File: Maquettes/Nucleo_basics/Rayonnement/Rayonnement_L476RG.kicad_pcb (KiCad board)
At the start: 2 copper layers, 120 x 110 mm, 48 parts, among them CON1 MikroE-Accelero, CON2 MikroE-nRF-S-module, J1 Speed_R, J10 Morpho_Gauche, J11 Morpho_Droite, J12 LED_1, J13 LED_2, J14 LED_3, J15 LED_4, J17 I2C_Visu, J18 I2C_EXT, J19 GND_reg, J2 Speed_L, J20 3.3V_reg, J21 MOT_R, J22 MOT_L, J23 D_IN_OUT, J3 Line_R, J4 Line_C, J5 Line_L, J6 US_Sensor, J7 Servo, J8 BAT_IN, J9 TC74A2-TempI2C, SW1 SW_1, SW2 SW_2, U1 MCP9700-Temp, U2 LM7805_TO220, U3 SN754410NE

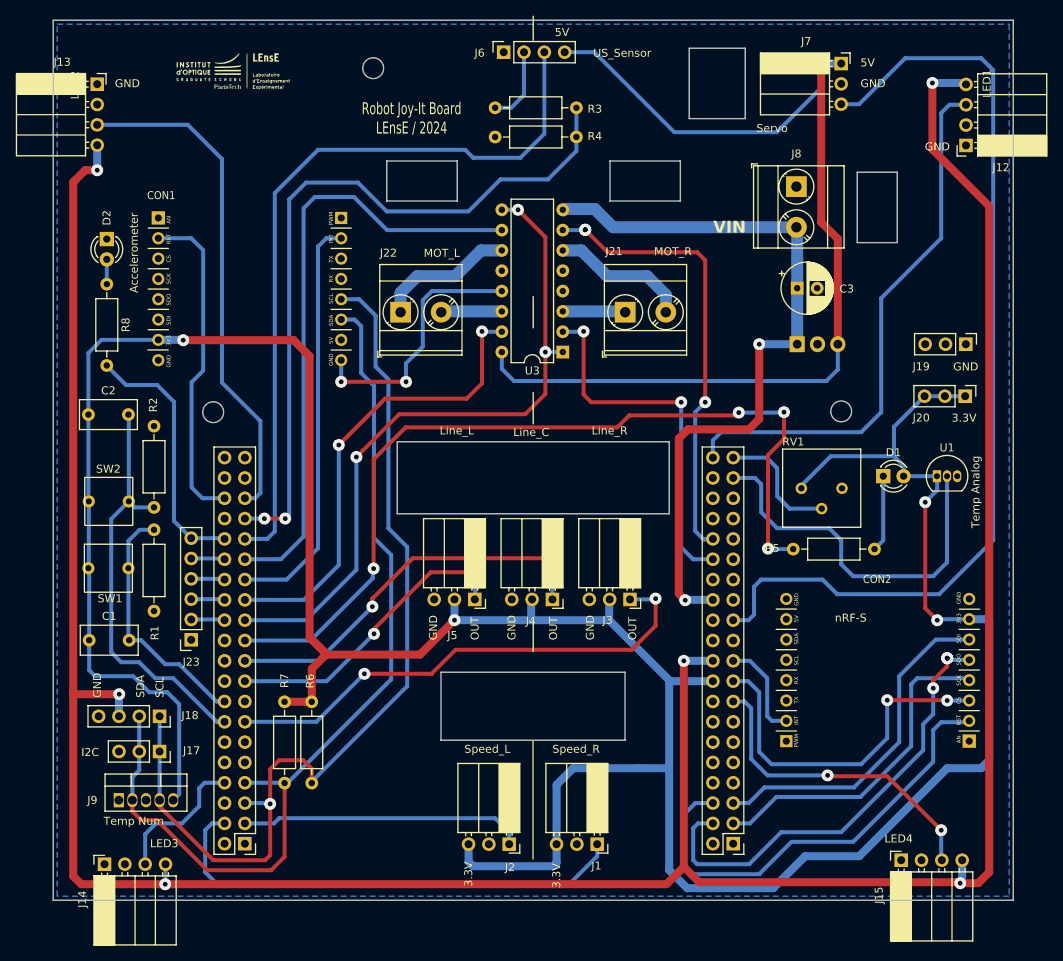
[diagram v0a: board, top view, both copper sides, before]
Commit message: Update Rayonnement
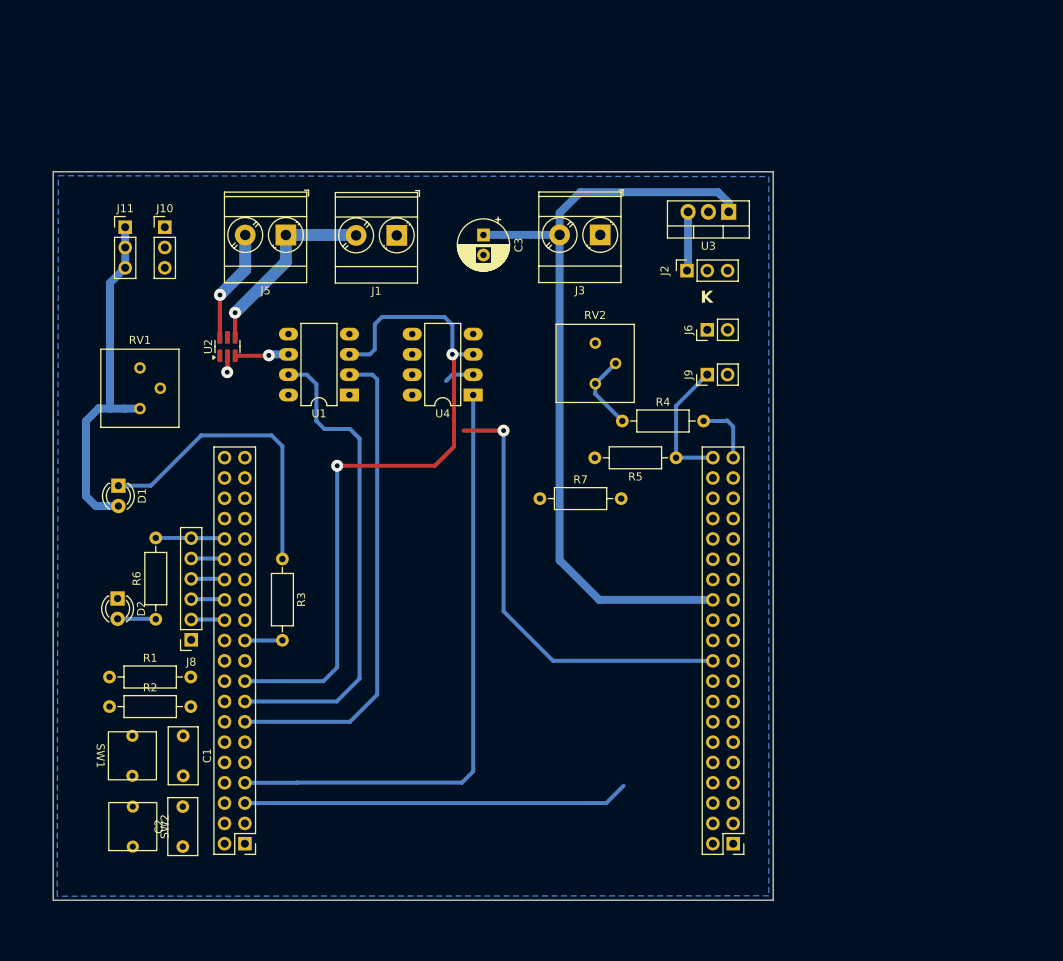
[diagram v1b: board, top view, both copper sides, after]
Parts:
- removed ? (x2): , 
- removed CON1: MikroE-Accelero, mikroE:MIKROBUS_MODULE_CONN
- removed CON2: MikroE-nRF-S-module, mikroE:MIKROBUS_MODULE_CONN
- removed G***: LOGO, LEnsE:Logo_Small
- removed J12: LED_1, Connector_PinSocket_2.54mm:PinSocket_1x04_P2.54mm_Horizontal
- removed J13: LED_2, Connector_PinSocket_2.54mm:PinSocket_1x04_P2.54mm_Horizontal
- removed J14: LED_3, Connector_PinSocket_2.54mm:PinSocket_1x04_P2.54mm_Horizontal
- removed J15: LED_4, Connector_PinSocket_2.54mm:PinSocket_1x04_P2.54mm_Horizontal
- removed J17: I2C_Visu, Connector_PinSocket_2.54mm:PinSocket_1x03_P2.54mm_Vertical
- removed J18: I2C_EXT, Connector_PinSocket_2.54mm:PinSocket_1x04_P2.54mm_Vertical
- removed J19: GND_reg, Connector_PinHeader_2.54mm:PinHeader_1x03_P2.54mm_Vertical
- removed J20: 3.3V_reg, Connector_PinHeader_2.54mm:PinHeader_1x03_P2.54mm_Vertical
- removed J21: MOT_R, TerminalBlock_Phoenix:TerminalBlock_Phoenix_MKDS-3-2-5.08_1x02_P5.08mm_Horizontal
- removed J22: MOT_L, TerminalBlock_Phoenix:TerminalBlock_Phoenix_MKDS-3-2-5.08_1x02_P5.08mm_Horizontal
- removed the J4 at (185.9, 112.9)
- removed the J7 at (222.0, 45.9)
- removed the J8 at (216.4, 61.3)
- removed R8: 100, Resistor_THT:R_Axial_DIN0207_L6.3mm_D2.5mm_P10.16mm_Horizontal
- removed REF** (x2): MountingHole_2.2mm_M2, MountingHole:MountingHole_2.2mm_M2
- added J10: GND_reg, Connector_PinHeader_2.54mm:PinHeader_1x03_P2.54mm_Vertical, F.Cu at (137.4, 66.4)
- added J11: 3.3V_reg, Connector_PinHeader_2.54mm:PinHeader_1x03_P2.54mm_Vertical, F.Cu at (132.5, 66.4)
- added RV2: 100k, Potentiometer_THT:Potentiometer_Bourns_3386P_Vertical, F.Cu at (191.3, 85.9)
- added U4: ~, Package_DIP:DIP-8_W7.62mm_LongPads, F.Cu at (176.0, 87.3)
- J1: value Speed_R -> LED_IN; footprint Connector_PinSocket_2.54mm:PinSocket_1x03_P2.54mm_Horizontal -> TerminalBlock_Phoenix:TerminalBlock_Phoenix_MKDS-3-2-5.08_1x02_P5.08mm_Horizontal
- J2: value Speed_L -> Servo; footprint Connector_PinSocket_2.54mm:PinSocket_1x03_P2.54mm_Horizontal -> Connector_PinSocket_2.54mm:PinSocket_1x03_P2.54mm_Vertical
- J3: value Line_R -> POWER_IN; footprint Connector_PinSocket_2.54mm:PinSocket_1x03_P2.54mm_Horizontal -> TerminalBlock_Phoenix:TerminalBlock_Phoenix_MKDS-3-2-5.08_1x02_P5.08mm_Horizontal
- J5: value Line_L -> LED_OUT; footprint Connector_PinSocket_2.54mm:PinSocket_1x03_P2.54mm_Horizontal -> TerminalBlock_Phoenix:TerminalBlock_Phoenix_MKDS-3-2-5.08_1x02_P5.08mm_Horizontal
- J6: value US_Sensor -> PhotoDiode; footprint Connector_PinSocket_2.54mm:PinSocket_1x04_P2.54mm_Vertical -> Connector_PinHeader_2.54mm:PinHeader_1x02_P2.54mm_Vertical
- J9: value TC74A2-TempI2C -> Thermistance; footprint Package_TO_SOT_THT:TO-220-5_Vertical -> Connector_PinHeader_2.54mm:PinHeader_1x02_P2.54mm_Vertical
- R3: value 2.2k -> 100
- R4: value 3.3k -> 100k
- R5: value 100 -> 10k
- R6: value 680 -> 100
- R7: value 680 -> 1k
- U1: value MCP9700-Temp -> ~; footprint Package_TO_SOT_THT:TO-92_Inline -> Package_DIP:DIP-8_W7.62mm_LongPads
- U2: value LM7805_TO220 -> BCR430UW6; footprint Package_TO_SOT_THT:TO-220-3_Vertical -> Package_TO_SOT_SMD:SC-74-6_1.55x2.9mm_P0.95mm; moved to F.Cu
- U3: value SN754410NE -> LM7805_TO220; footprint Package_DIP:DIP-16_W7.62mm -> Package_TO_SOT_THT:TO-220-3_Vertical
- moved D1 95.6 mm to (131.7, 98.7), turned to -90 degrees
- moved J9 90.8 mm to (205.3, 84.8), turned to 90 degrees
- moved RV1 83.3 mm to (134.3, 89.0), turned to 0 degrees
- moved J1 80.1 mm to (166.4, 67.4), turned to 180 degrees
- moved J2 75.1 mm to (202.7, 71.8), turned to 90 degrees
- moved U1 74.1 mm to (160.5, 87.3), turned to 180 degrees
- moved U2 71.2 mm to (145.3, 81.3), turned to 90 degrees
- moved R3 67.3 mm to (152.2, 107.8), turned to -90 degrees
- moved C2 55.3 mm to (139.7, 143.8), turned to 90 degrees
- moved J5 51.3 mm to (152.6, 67.3), turned to 180 degrees
- moved J3 45.7 mm to (191.9, 67.3), turned to 180 degrees
- moved D2 45.0 mm to (131.6, 112.8)
- moved J6 43.0 mm to (205.3, 79.2)
- moved R7 40.8 mm to (184.3, 100.3), turned to 0 degrees
- moved C3 39.8 mm to (177.3, 67.3), turned to -90 degrees
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- renumbered J10 to J4, J11 to J7, J23 to J8
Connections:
- J1 pad 1: Speed_R -> GND
- J1 pad 2: GND -> LED_POW_IN
- J2 pad 1: Speed_L -> 5V
- J2 pad 3: 3.3V_NUC -> Servo
- J3 pad 1: Line_R -> GND
- J3 pad 2: 3.3V_NUC -> VIN
- J4 pad 15: Din_4 -> unconnected-(J4-Pin_15-Pad15)
- J4 pad 17: nRF_CS -> unconnected-(J4-Pin_17-Pad17)
- J4 pad 19: nRF_INT -> unconnected-(J4-Pin_19-Pad19)
- J4 pad 23: Servo -> unconnected-(J4-Pin_23-Pad23)
- J4 pad 3: SCK -> unconnected-(J4-Pin_3-Pad3)
- J4 pad 30: MOT_R_1 -> POT_OUT
- J4 pad 32: MOT_R_2 -> unconnected-(J4-Pin_32-Pad32)
- J4 pad 34: ADC_OUT -> unconnected-(J4-Pin_34-Pad34)
- J4 pad 36: unconnected-(J10-Pin_36-Pad36) -> POT_NUM_OUT
- J4 pad 37: TEMP_OUT -> unconnected-(J4-Pin_37-Pad37)
- J4 pad 39: POT_OUT -> PHD_OUT
- J4 pad 4: MISO -> unconnected-(J4-Pin_4-Pad4)
- J4 pad 40: Din_1 -> RT_OUT
- J4 pad 5: MOSI -> unconnected-(J4-Pin_5-Pad5)
- J4 pad 6: nRF_CE -> unconnected-(J4-Pin_6-Pad6)
- J5 pad 1: Line_L -> LED_POW_IN
- J5 pad 2: 3.3V_NUC -> Net-(J5-Pin_2)
- J6 pad 1: GND -> 3.3V_NUC
- J6 pad 2: US_echo -> PHD_OUT
- J7 pad 13: Line_R -> SCK
- J7 pad 14: SW2_OUT -> unconnected-(J7-Pin_14-Pad14)
- J7 pad 15: unconnected-(J11-Pin_15-Pad15) -> MISO
- J7 pad 16: SW1_OUT -> unconnected-(J7-Pin_16-Pad16)
- J7 pad 17: Line_L -> MOSI
- J7 pad 19: Line_C -> unconnected-(J7-Pin_19-Pad19)
- J7 pad 23: MOT_EN -> unconnected-(J7-Pin_23-Pad23)
- J7 pad 25: MOT_L_2 -> unconnected-(J7-Pin_25-Pad25)
- J7 pad 27: Accel_INT -> unconnected-(J7-Pin_27-Pad27)
- J7 pad 29: MOT_L_1 -> unconnected-(J7-Pin_29-Pad29)
- J7 pad 3: Speed_L -> unconnected-(J7-Pin_3-Pad3)
- J7 pad 31: US_trig -> CS_1
- J7 pad 33: US_echo_in -> unconnected-(J7-Pin_33-Pad33)
- J7 pad 35: Din_2 -> unconnected-(J7-Pin_35-Pad35)
- J7 pad 36: Accel_RESET -> unconnected-(J7-Pin_36-Pad36)
- J7 pad 4: Speed_R -> SW2_OUT
- J7 pad 5: SCL -> Servo
- J7 pad 6: unconnected-(J11-Pin_6-Pad6) -> SW1_OUT
- J7 pad 7: SDA -> CS_2
- J7 pad 8: Din_3 -> unconnected-(J7-Pin_8-Pad8)
- J9 pad 1: unconnected-(J9-Pin_1-Pad1) -> RT_OUT
- J9 pad 2: SDA -> GND
- R3 pad 1: US_echo_in -> Net-(D1-K)
- R3 pad 2: US_echo -> LED_OUT
- R4 pad 1: GND -> Net-(R4-Pad1)
- R4 pad 2: US_echo_in -> PHD_OUT
- R5 pad 1: Net-(D1-K) -> RT_OUT
- R5 pad 2: LED_OUT -> 3.3V_NUC
- R6 pad 1: 3.3V_NUC -> Net-(D2-A)
- R6 pad 2: SCL -> LED_OUT2
- R7 pad 1: 3.3V_NUC -> POT_NUM_OUT
- R7 pad 2: SDA -> GND
- U1 pad 1: 3.3V_NUC -> CS_1
- U1 pad 2: TEMP_OUT -> SCK
- U1 pad 3: GND -> MOSI
- U2 pad 1: VIN -> unconnected-(U2-NC-Pad1)
- U2 pad 3: 5V -> Net-(U1-POB)
- U3 pad 1: MOT_EN -> VIN
- U3 pad 2: MOT_R_1 -> GND
- U3 pad 3: Net-(J21-Pin_1) -> 5V
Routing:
- net 3.3V_NUC: track 393.8 -> 44.9 mm, vias 4 -> 0
- net 5V_NUC: track 360.1 -> 56.3 mm, vias 6 -> 1
- net 5V: track 128.8 -> 7.40 mm, vias 1 -> 0
- net SCL: track 120.2 -> 0.00 mm, vias 1 -> 0
- net SDA: track 116.6 -> 0.00 mm
- net LED_OUT: track 109.0 -> 4.70 mm, vias 4 -> 0
- net US_trig: track 94.2 -> 0.00 mm
- net US_echo_in: track 91.9 -> 0.00 mm, vias 2 -> 0
- net MOT_EN: track 86.2 -> 0.00 mm, vias 3 -> 0
- net MOT_L_1: track 76.6 -> 0.00 mm
- net CS_2: track 0.00 -> 76.2 mm
- net Servo: track 120.9 -> 48.2 mm
- net Din_1: track 68.7 -> 0.00 mm
- net Din_2: track 63.3 -> 0.00 mm
- net Line_R: track 63.0 -> 0.00 mm, vias 2 -> 0
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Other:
- board size 120 x 110 mm -> 90 x 91 mm
- board text added: "K"
- board text removed: "${REFERENCE}"
- board text removed: "3.3V"
- board text removed: "5V"
- board text removed: "Accelerometer"
- board text removed: "GND"
- board text removed: "I2C"
- board text removed: "LED1"
- board text removed: "LED2"
- board text removed: "LED3"
- board text removed: "LED4"
- board text removed: "Line_C"
- board text removed: "Line_L"
- board text removed: "Line_R"
- board text removed: "MOT_L"
- board text removed: "MOT_R"
- board text removed: "OUT"
- board text removed: "Robot Joy-It Board LEnsE / 2024"
- board text removed: "SCL"
- board text removed: "SDA"
- board text removed: "Servo"
- board text removed: "Speed_L"
- board text removed: "Speed_R"
- board text removed: "Temp Analog"
- board text removed: "Temp Num"
- board text removed: "US_Sensor"
- board text removed: "VIN"
- board text removed: "nRF-S"
